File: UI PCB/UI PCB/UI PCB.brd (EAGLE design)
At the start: 67.3 x 50.5 mm, 23 parts, among them IC1 MCP23S17SP, IC2 MCP23S17SP, X1 JST-XH-02-PIN-ROUND-PAD, X2 JST-XH-02-PIN-ROUND-PAD, X3 JST-XH-02-PIN-ROUND-PAD, X4 JST-XH-02-PIN-ROUND-PAD, X5 JST-XH-05-PIN-ROUND-PAD, X6 JST-XH-05-PIN-ROUND-PAD, X7 JST-XH-05-PIN-ROUND-PAD, X8 JST-XH-05-PIN-ROUND-PAD, X9 JST-XH-05-PIN-ROUND-PAD

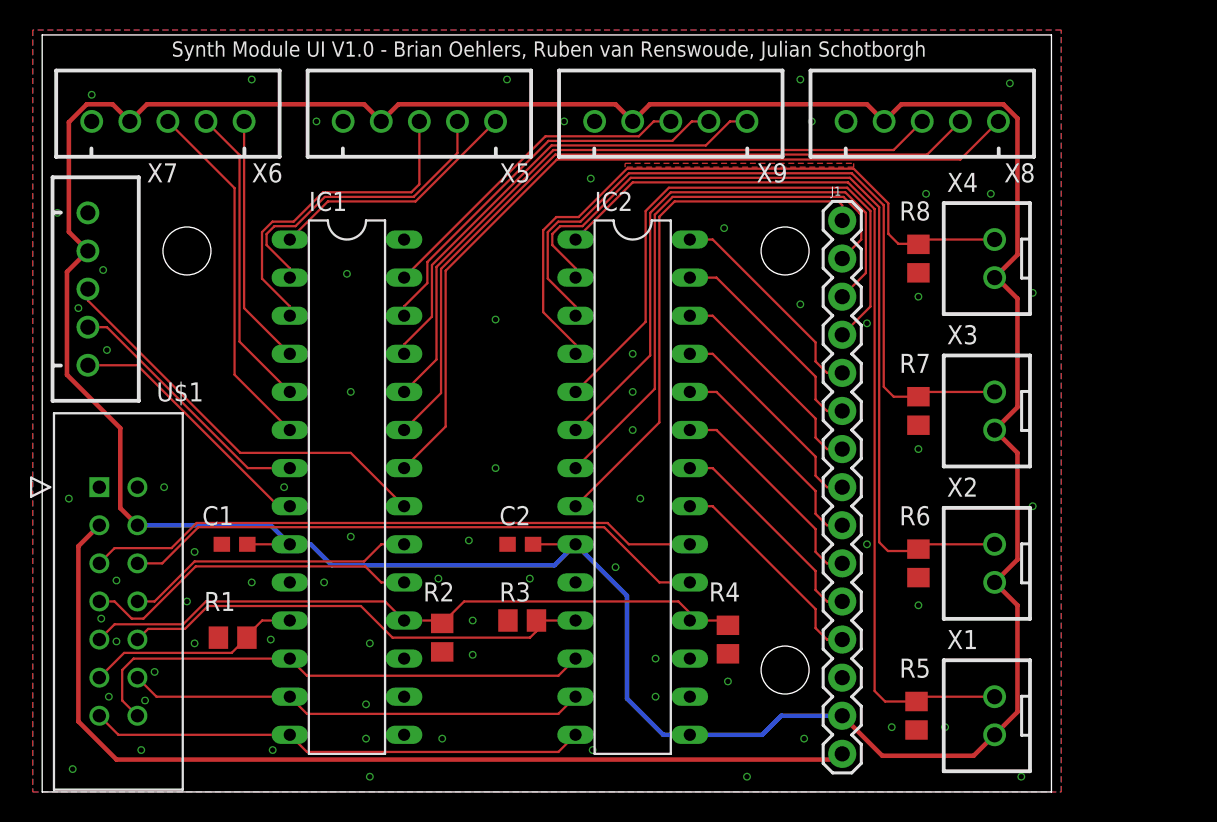
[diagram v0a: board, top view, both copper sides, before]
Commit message: gerber files toegevoegd
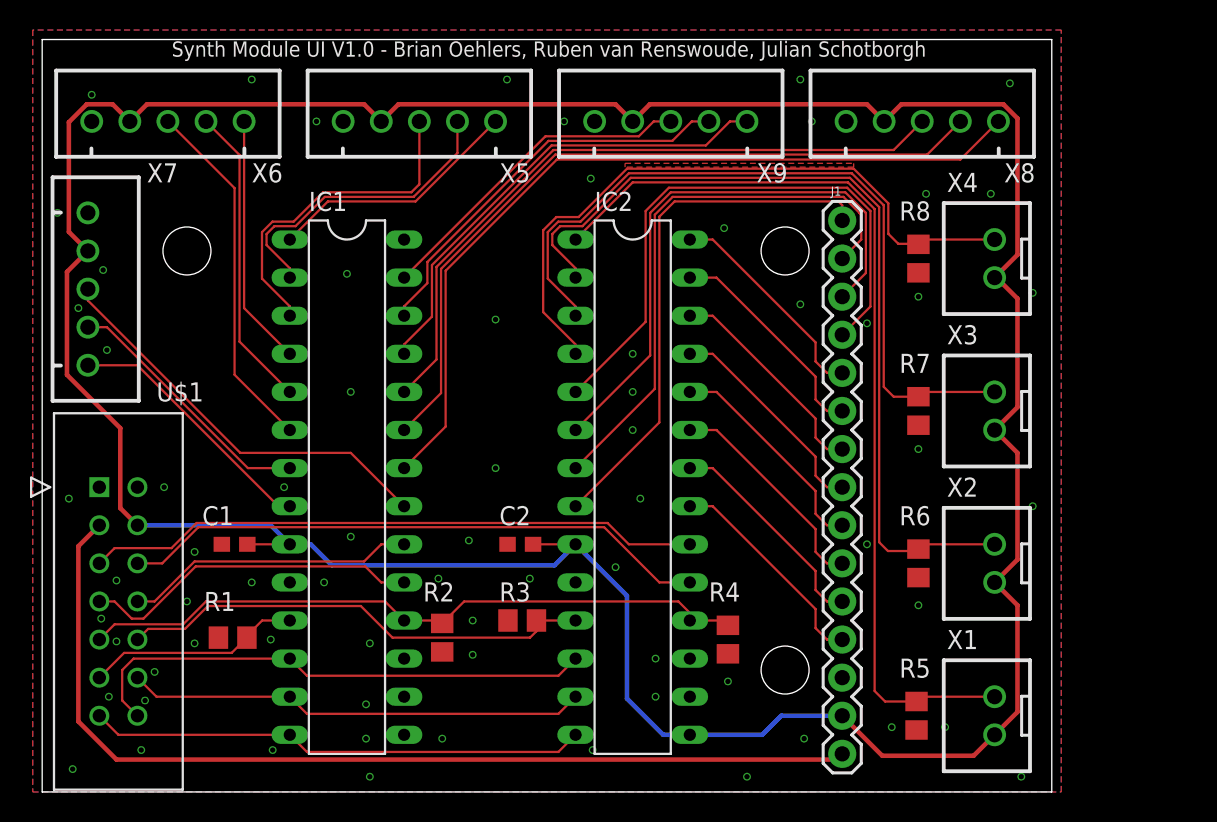
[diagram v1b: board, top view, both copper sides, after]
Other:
- board size 67.3 x 50.5 mm -> 67.3 x 50.2 mm
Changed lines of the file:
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@@
 <?xml version="1.0" encoding="utf-8"?>
 <!DOCTYPE eagle SYSTEM "eagle.dtd">
-<eagle version="9.5.1">
+<eagle version="9.5.2">
 <drawing>
 <settings>
@@
 <board>
 <plain>
-<wire x1="0" y1="0" x2="67.29" y2="0" width="0" layer="20"/>
-<wire x1="67.29" y1="0" x2="67.29" y2="50.47" width="0" layer="20"/>
-<wire x1="67.29" y1="50.47" x2="0" y2="50.47" width="0" layer="20"/>
-<wire x1="0" y1="50.47" x2="0" y2="0" width="0" layer="20"/>
+<wire x1="0" y1="0" x2="67.31" y2="0" width="0" layer="20"/>
+<wire x1="67.31" y1="0" x2="67.31" y2="50.165" width="0" layer="20"/>
+<wire x1="67.31" y1="50.165" x2="0" y2="50.165" width="0" layer="20"/>
+<wire x1="0" y1="50.165" x2="0" y2="0" width="0" layer="20"/>
 <hole x="9.652" y="36.068" drill="3.2"/>
 <hole x="49.53" y="36.068" drill="3.2"/>
 <hole x="49.53" y="8.128" drill="3.2"/>
 <text x="8.636" y="49.022" size="1.016" layer="25">Synth Module UI V1.0 - Brian Oehlers, Ruben van Renswoude, Julian Schotborgh</text>
-<dimension x1="43.18" y1="36.83" x2="43.18" y2="34.29" x3="69.215" y3="35.56" textsize="1.778" layer="1"/>
-<dimension x1="43.18" y1="34.29" x2="43.18" y2="31.75" x3="73.025" y3="33.02" textsize="1.778" layer="1"/>
-<dimension x1="43.18" y1="29.21" x2="43.18" y2="31.75" x3="76.835" y3="30.48" textsize="1.778" layer="1"/>
-<dimension x1="43.18" y1="29.21" x2="43.18" y2="26.67" x3="82.55" y3="27.94" textsize="1.778" layer="1"/>
-<dimension x1="43.18" y1="3.81" x2="43.18" y2="36.83" x3="92.71" y3="20.32" textsize="1.778" layer="1"/>
-<dimension x1="43.18" y1="24.13" x2="43.18" y2="26.67" x3="79.375" y3="25.4" textsize="1.778" layer="1"/>
 <dimension x1="67.29" y1="50.47" x2="0" y2="50.47" x3="33.645" y3="54.61" textsize="1.778" layer="1"/>
 </plain>
